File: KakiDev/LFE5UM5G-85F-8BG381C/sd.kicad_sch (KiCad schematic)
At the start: 3 parts, among them J6 Micro_SD_Card_Det2, U1 ECP5-CABGA256

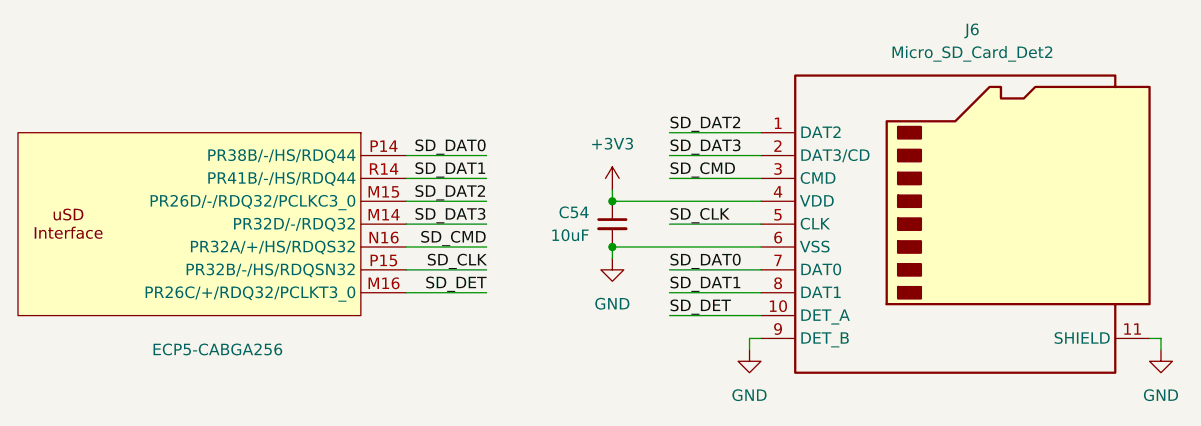
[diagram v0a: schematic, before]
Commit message: jkfjhaqju
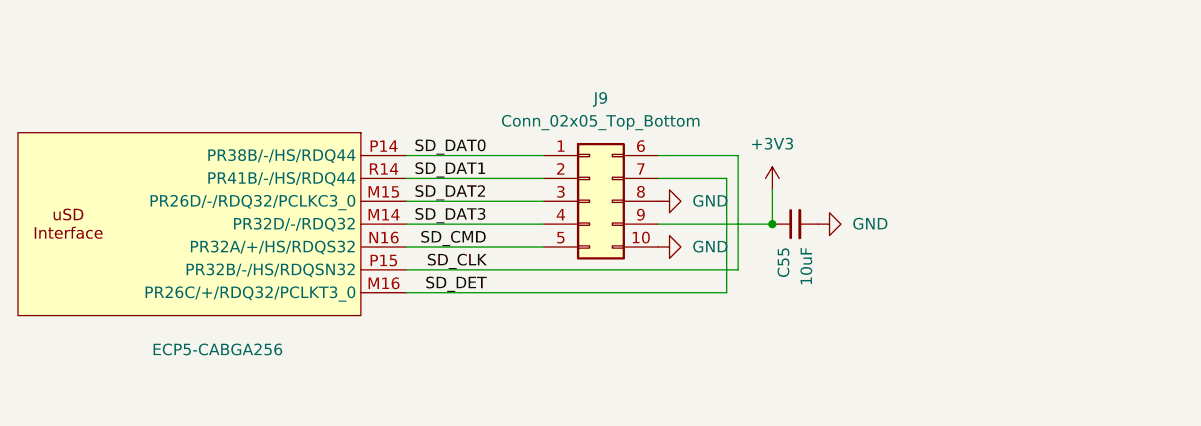
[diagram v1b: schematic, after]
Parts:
- removed C54: 10uF, Capacitor_SMD:C_0603_1608Metric, symbol Device:C_Small
- removed J6: Micro_SD_Card_Det2, icepi-lib:microSD_HC_SOFNG_TF-008, symbol Connector:Micro_SD_Card_Det2
- added C55: 10uF, Capacitor_SMD:C_0603_1608Metric, symbol Device:C_Small
- added J9: Conn_02x05_Top_Bottom, Connector_PinHeader_2.54mm:PinHeader_2x05_P2.54mm_Vertical, symbol Connector_Generic:Conn_02x05_Top_Bottom
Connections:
- net +3V3: now also C55.1, J9.9 (Pin_9)
- net GND: now also C55.2, J9.10 (Pin_10), J9.8 (Pin_8)
- net SD_CLK: now also J9.6 (Pin_6)
- net SD_CMD: now also J9.5 (Pin_5)
- net SD_DAT0: now also J9.1 (Pin_1)
- net SD_DAT1: now also J9.2 (Pin_2)
- net SD_DAT2: now also J9.3 (Pin_3)
- net SD_DAT3: now also J9.4 (Pin_4)
- net SD_DET: now also J9.7 (Pin_7)
